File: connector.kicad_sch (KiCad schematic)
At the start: 4 parts, among them J6 Conn_01x90_3Row_Header

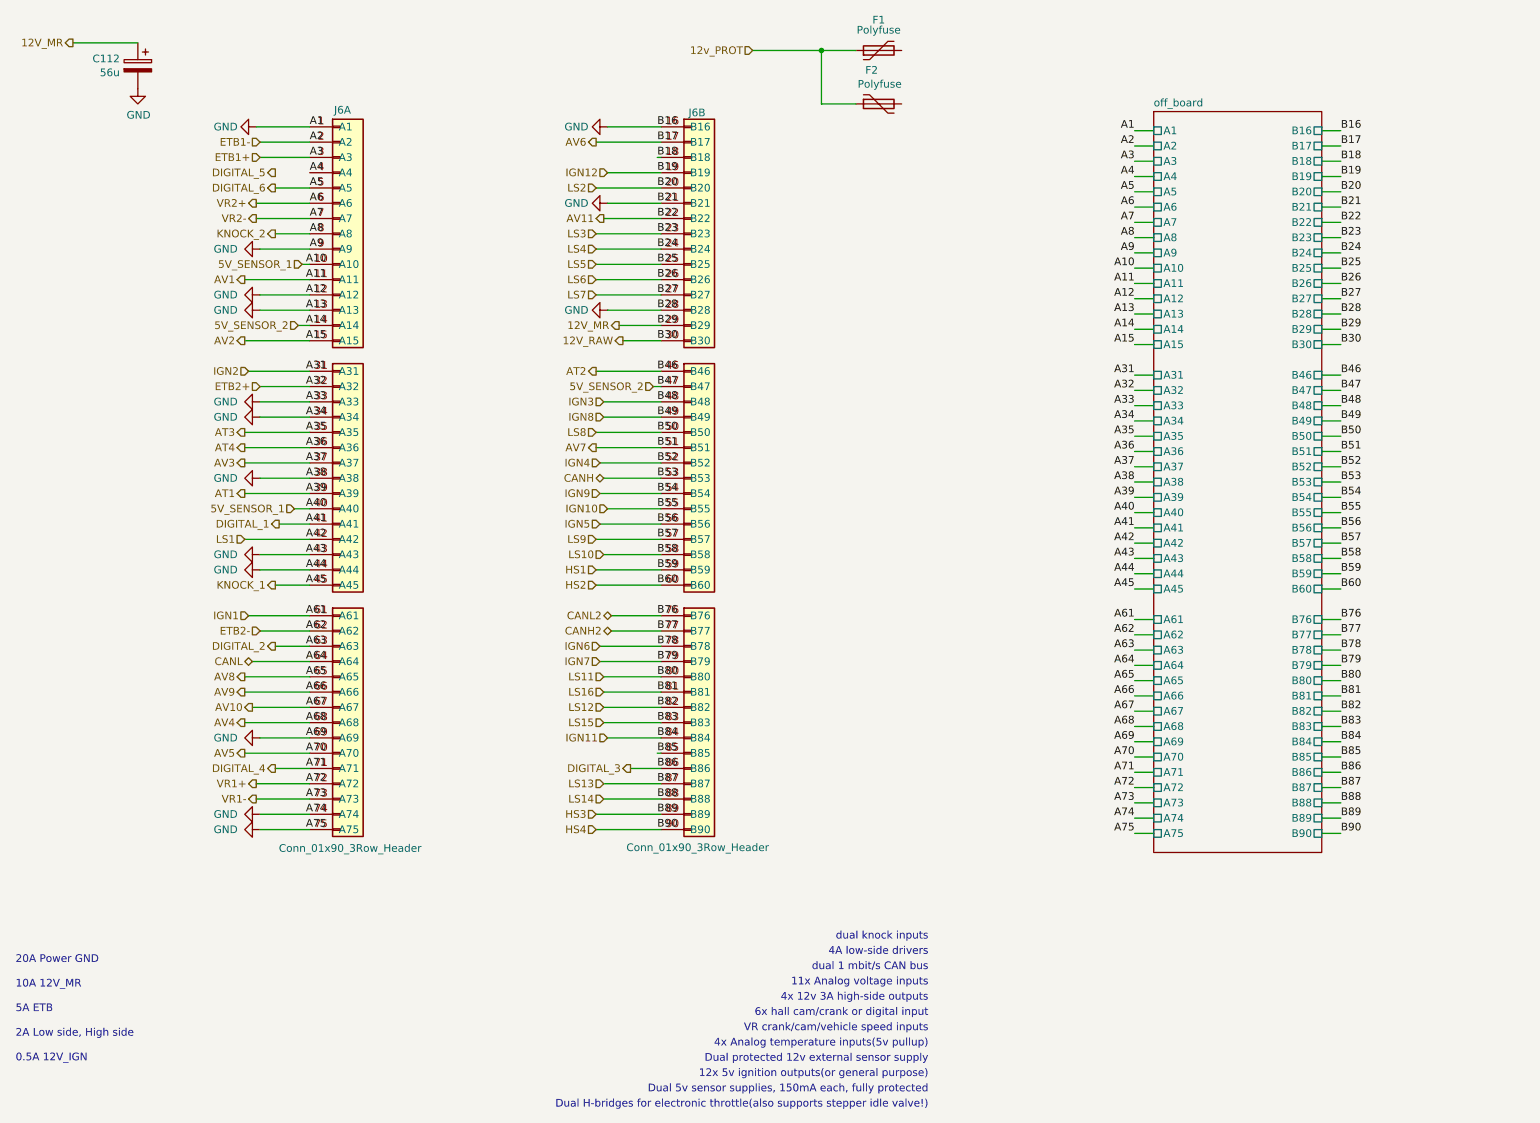
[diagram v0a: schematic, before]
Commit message: external loops
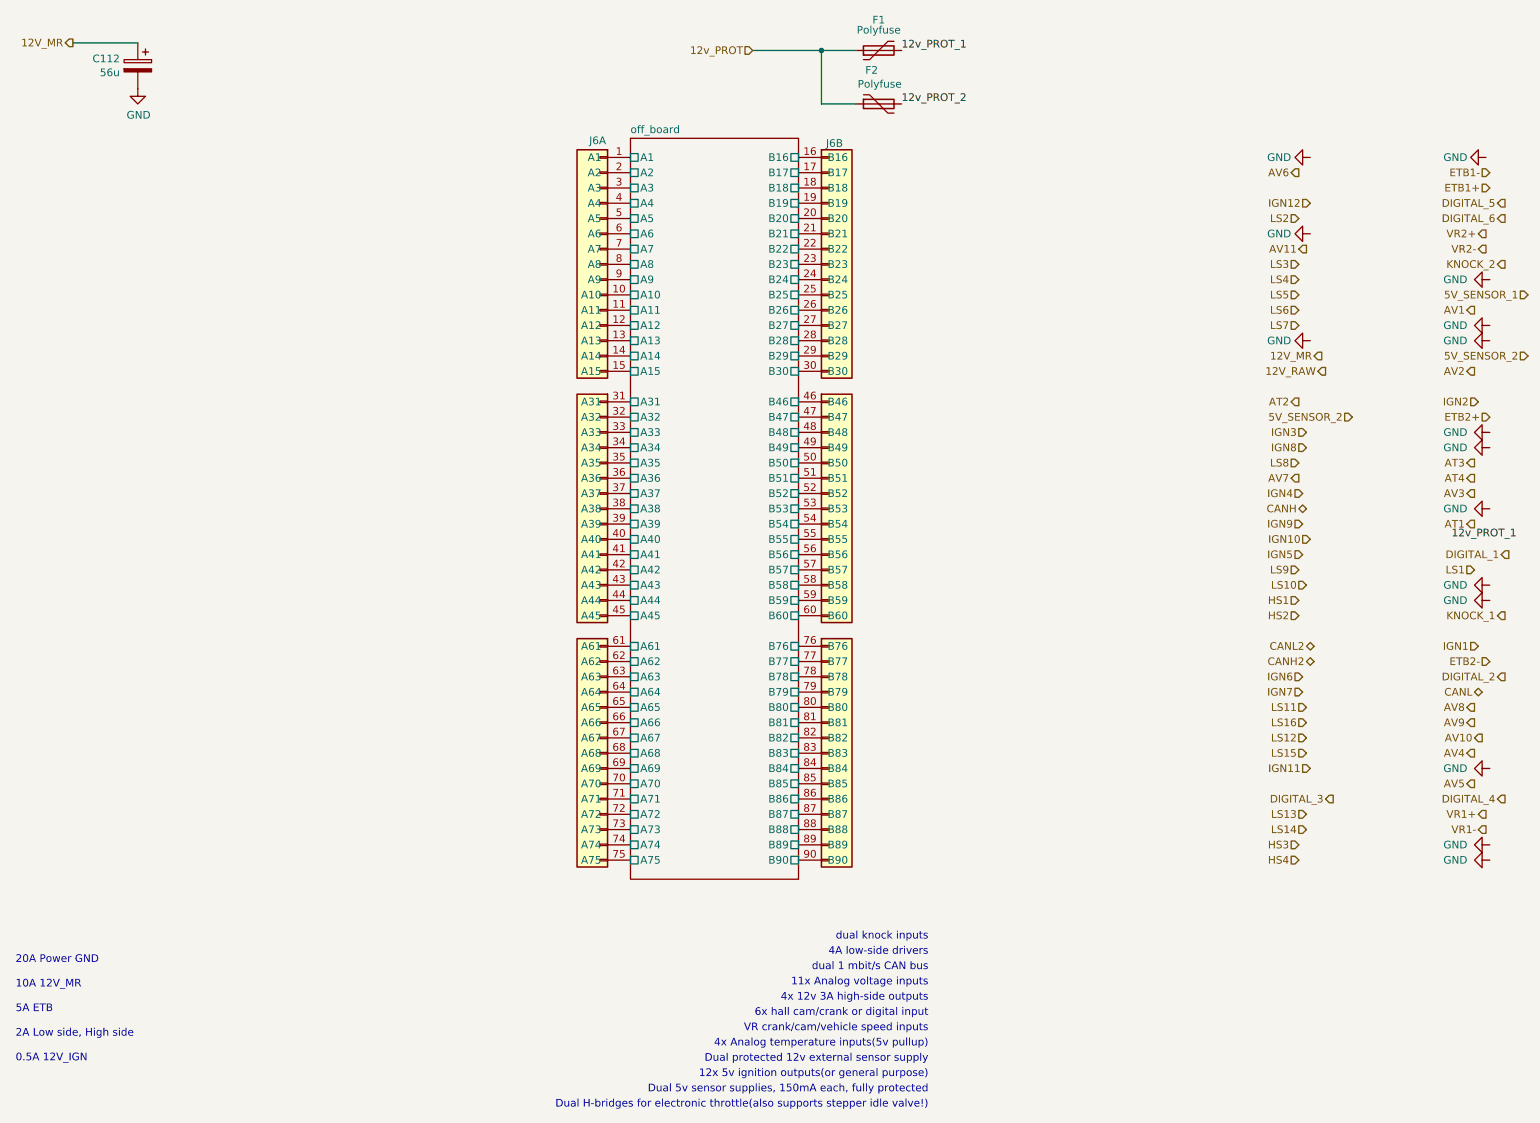
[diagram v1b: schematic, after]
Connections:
- net 12V_MR: no longer J6.29 (B29)
- net 12V_RAW: no longer J6.30 (B30)
- net 5V_SENSOR_1: no longer J6.10 (A10), J6.40 (A40)
- net 5V_SENSOR_2: no longer J6.14 (A14), J6.47 (B47)
- net AT1: no longer J6.39 (A39)
- net AT2: no longer J6.46 (B46)
- net AT3: no longer J6.35 (A35)
- net AT4: no longer J6.36 (A36)
- net AV1: no longer J6.11 (A11)
- net AV10: no longer J6.67 (A67)
- net AV11: no longer J6.22 (B22)
- net AV2: no longer J6.15 (A15)
- net AV3: no longer J6.37 (A37)
- net AV4: no longer J6.68 (A68)
- net AV5: no longer J6.70 (A70)
- net AV6: no longer J6.17 (B17)
- net AV7: no longer J6.51 (B51)
- net AV8: no longer J6.65 (A65)
- net AV9: no longer J6.66 (A66)
- net CANH: no longer J6.53 (B53)
- net CANH2: no longer J6.77 (B77)
- net CANL: no longer J6.64 (A64)
- net CANL2: no longer J6.76 (B76)
- net DIGITAL_1: no longer J6.41 (A41)
- net DIGITAL_2: no longer J6.63 (A63)
- net DIGITAL_3: no longer J6.86 (B86)
- net DIGITAL_4: no longer J6.71 (A71)
- net DIGITAL_6: no longer J6.5 (A5)
- net ETB1+: no longer J6.3 (A3)
- net ETB1-: no longer J6.2 (A2)
- net ETB2+: no longer J6.32 (A32)
- net ETB2-: no longer J6.62 (A62)
- net GND: no longer J6.1 (A1), J6.12 (A12), J6.13 (A13), J6.16 (B16), J6.21 (B21), J6.28 (B28), J6.33 (A33), J6.34 (A34), J6.38 (A38), J6.43 (A43), J6.44 (A44), J6.69 (A69), J6.74 (A74), J6.75 (A75), J6.9 (A9)
- net HS1: no longer J6.59 (B59)
- net HS2: no longer J6.60 (B60)
- net HS3: no longer J6.89 (B89)
- net HS4: no longer J6.90 (B90)
- net IGN1: no longer J6.61 (A61)
- net IGN10: no longer J6.55 (B55)
- net IGN11: no longer J6.84 (B84)
- net IGN12: no longer J6.19 (B19)
- net IGN2: no longer J6.31 (A31)
- net IGN3: no longer J6.48 (B48)
- net IGN4: no longer J6.52 (B52)
- net IGN5: no longer J6.56 (B56)
- net IGN6: no longer J6.78 (B78)
- net IGN7: no longer J6.79 (B79)
- net IGN8: no longer J6.49 (B49)
- net IGN9: no longer J6.54 (B54)
- net KNOCK_1: no longer J6.45 (A45)
- net KNOCK_2: no longer J6.8 (A8)
- net LS1: no longer J6.42 (A42)
- net LS10: no longer J6.58 (B58)
- net LS11: no longer J6.80 (B80)
- net LS12: no longer J6.82 (B82)
- net LS13: no longer J6.87 (B87)
- net LS14: no longer J6.88 (B88)
- net LS15: no longer J6.83 (B83)
- net LS16: no longer J6.81 (B81)
- net LS2: no longer J6.20 (B20)
- net LS3: no longer J6.23 (B23)
- net LS4: no longer J6.24 (B24)
- net LS5: no longer J6.25 (B25)
- net LS6: no longer J6.26 (B26)
- net LS7: no longer J6.27 (B27)
- net LS8: no longer J6.50 (B50)
- net LS9: no longer J6.57 (B57)
- net VR1+: no longer J6.72 (A72)
- net VR1-: no longer J6.73 (A73)
- net VR2+: no longer J6.6 (A6)
- net VR2-: no longer J6.7 (A7)
- net 12v_PROT_2: now reaches F2.2
- net 12v_PROT_1: now reaches F1.2
- net A4 renamed off_board/A4
- net B18 renamed off_board/B18
- net B85 renamed off_board/B85
- new net off_board/A1: J6.1 (A1)
- new net off_board/A10: J6.10 (A10)
- new net off_board/A11: J6.11 (A11)
- new net off_board/A12: J6.12 (A12)
- new net off_board/A13: J6.13 (A13)
- new net off_board/A14: J6.14 (A14)
- new net off_board/A15: J6.15 (A15)
- new net off_board/A2: J6.2 (A2)
- new net off_board/A3: J6.3 (A3)
- new net off_board/A31: J6.31 (A31)
- new net off_board/A32: J6.32 (A32)
- new net off_board/A33: J6.33 (A33)
- new net off_board/A34: J6.34 (A34)
- new net off_board/A35: J6.35 (A35)
- new net off_board/A36: J6.36 (A36)
- new net off_board/A37: J6.37 (A37)
- new net off_board/A38: J6.38 (A38)
- new net off_board/A39: J6.39 (A39)
- new net off_board/A40: J6.40 (A40)
- new net off_board/A41: J6.41 (A41)
- new net off_board/A42: J6.42 (A42)
- new net off_board/A43: J6.43 (A43)
- new net off_board/A44: J6.44 (A44)
- new net off_board/A45: J6.45 (A45)
- new net off_board/A5: J6.5 (A5)
- new net off_board/A6: J6.6 (A6)
- new net off_board/A61: J6.61 (A61)
- new net off_board/A62: J6.62 (A62)
- new net off_board/A63: J6.63 (A63)
- new net off_board/A64: J6.64 (A64)
- new net off_board/A65: J6.65 (A65)
- new net off_board/A66: J6.66 (A66)
- new net off_board/A67: J6.67 (A67)
- new net off_board/A68: J6.68 (A68)
- new net off_board/A69: J6.69 (A69)
- new net off_board/A7: J6.7 (A7)
- new net off_board/A70: J6.70 (A70)
- new net off_board/A71: J6.71 (A71)
- new net off_board/A72: J6.72 (A72)
- new net off_board/A73: J6.73 (A73)
- new net off_board/A74: J6.74 (A74)
- new net off_board/A75: J6.75 (A75)
- new net off_board/A8: J6.8 (A8)
- new net off_board/A9: J6.9 (A9)
- new net off_board/B16: J6.16 (B16)
- new net off_board/B17: J6.17 (B17)
- new net off_board/B19: J6.19 (B19)
- new net off_board/B20: J6.20 (B20)
- new net off_board/B21: J6.21 (B21)
- new net off_board/B22: J6.22 (B22)
- new net off_board/B23: J6.23 (B23)
- new net off_board/B24: J6.24 (B24)
- new net off_board/B25: J6.25 (B25)
- new net off_board/B26: J6.26 (B26)
- new net off_board/B27: J6.27 (B27)
- new net off_board/B28: J6.28 (B28)
- new net off_board/B29: J6.29 (B29)
- new net off_board/B30: J6.30 (B30)
- new net off_board/B46: J6.46 (B46)
- new net off_board/B47: J6.47 (B47)
- new net off_board/B48: J6.48 (B48)
- new net off_board/B49: J6.49 (B49)
- new net off_board/B50: J6.50 (B50)
- new net off_board/B51: J6.51 (B51)
- new net off_board/B52: J6.52 (B52)
- new net off_board/B53: J6.53 (B53)
- new net off_board/B54: J6.54 (B54)
- new net off_board/B55: J6.55 (B55)
- new net off_board/B56: J6.56 (B56)
- new net off_board/B57: J6.57 (B57)
- new net off_board/B58: J6.58 (B58)
- new net off_board/B59: J6.59 (B59)
- new net off_board/B60: J6.60 (B60)
- new net off_board/B76: J6.76 (B76)
- new net off_board/B77: J6.77 (B77)
- new net off_board/B78: J6.78 (B78)
- new net off_board/B79: J6.79 (B79)
- new net off_board/B80: J6.80 (B80)
- new net off_board/B81: J6.81 (B81)
- new net off_board/B82: J6.82 (B82)
- new net off_board/B83: J6.83 (B83)
- new net off_board/B84: J6.84 (B84)
- new net off_board/B86: J6.86 (B86)
- new net off_board/B87: J6.87 (B87)
- new net off_board/B88: J6.88 (B88)
- new net off_board/B89: J6.89 (B89)
- new net off_board/B90: J6.90 (B90)
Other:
- moved on the sheet: J6A

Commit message: external loops arrangments
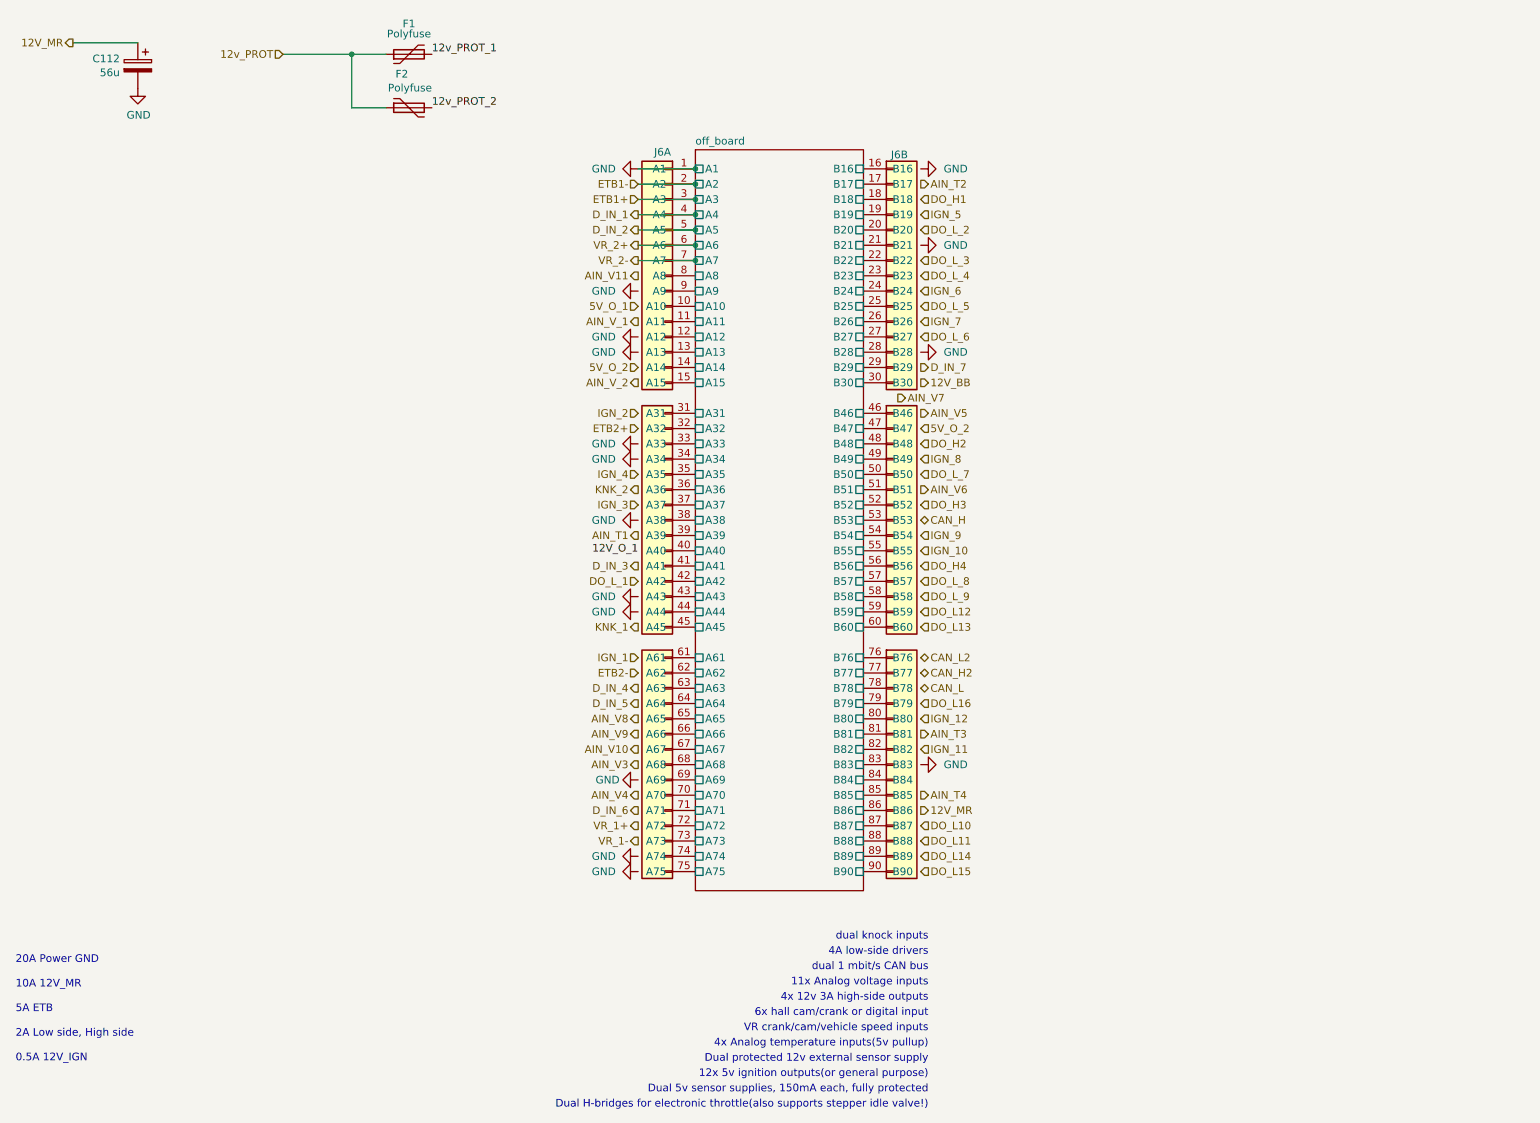
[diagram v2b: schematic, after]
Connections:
- net off_board/A1 is gone; now on net GND: J6.1 (A1)
- net off_board/A2 is gone; now on net ETB1-: J6.2 (A2)
- net off_board/A3 is gone; now on net ETB1+: J6.3 (A3)
- net off_board/A4 renamed D_IN_1
- net off_board/A5 renamed D_IN_2
- net off_board/A6 renamed VR_2+
- net off_board/A7 renamed VR_2-
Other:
- moved on the sheet: F1, F2, J6A, J6B
